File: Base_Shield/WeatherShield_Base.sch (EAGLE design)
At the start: 71 parts, among them Q1 BSS138, Q2 BSS138, U1 DS3231SN, U2 LT3652

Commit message: WeatherShield_v1
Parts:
- removed U$5: MCP3221A5T-E/OT, FSEWeatherShield:MCP3221A5T-E/OT
- added C5: 0.1uF, rcl:C-EUC0603
- added JP1, JP2, JP4: (no value), pinhead:PINHD-1X2
- added JP5: (no value), pinhead:PINHD-1X3
- added JP6, JP7, JP8: (no value), pinhead:PINHD-1X1
- added U3: TMP100MDBVREP, FSEWeatherShield:TMP100MDBVREP
- added U4: ADS1015IDGST, FSEWeatherShield:ADS1015IDGST
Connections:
- new net N$14: JP6.1, U4.AIN1
- new net N$18: JP4.1, PCB1.TXD0/GPIO14
- new net N$19: JP4.2, PCB1.RXD0/GPIO15
- new net N$20: JP5.3, PCB1.GPIO10/MOSI
- new net N$21: JP5.2, PCB1.GPIO09/MISO
- new net N$25: JP5.1, PCB1.GPIO11/SCLK
- new net N$8: JP7.1, U4.AIN2
- new net N$9: JP8.1, U4.AIN3
- net 3.3V: now also C5.1, JP2.1, U3.V+
- net 5V: now also JP1.1, U4.VDD; no longer C20.1, C21.1, U$5.VDD
- net GND: now also C5.2, JP1.2, JP2.2, U3.AD0, U3.AD1, U3.GND, U4.ADDR, U4.GND; no longer C20.2, C21.2, U$5.VSS
- net HV_SCL: now also U4.SCL; no longer PCB1.GPIO03/SCL1
- net HV_SDA: now also U4.SDA; no longer PCB1.GPIO02/SDA1
- net RAIN: now also PCB1.GPIO18
- net SCL: now also PCB1.GPIO03/SCL1, U3.SCL; no longer U$5.SCL
- net SDA: now also PCB1.GPIO02/SDA1, U3.SDA; no longer U$5.SDA
- net STAT3: now also PCB1.GPIO21
- net WDIR: now also U4.AIN0; no longer U$5.AIN
- net WSPEED: now also PCB1.GPIO17/GEN0
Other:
- note added: "7-Bit I2C Address is 0x48"
- note added: "7-Bit I2C Address is 0x68"
- note added: "Add. SPI"
- note added: "Add. UART"
- note added: "Air Board Interface"
- note added: "Level shifter"
- note added: "Solar cell"
- note added: "Temperatur sensor"
- moved on the sheet: C1, C10, C11, C12, C13, C14, C15, C16, C17, C18, C19, C2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

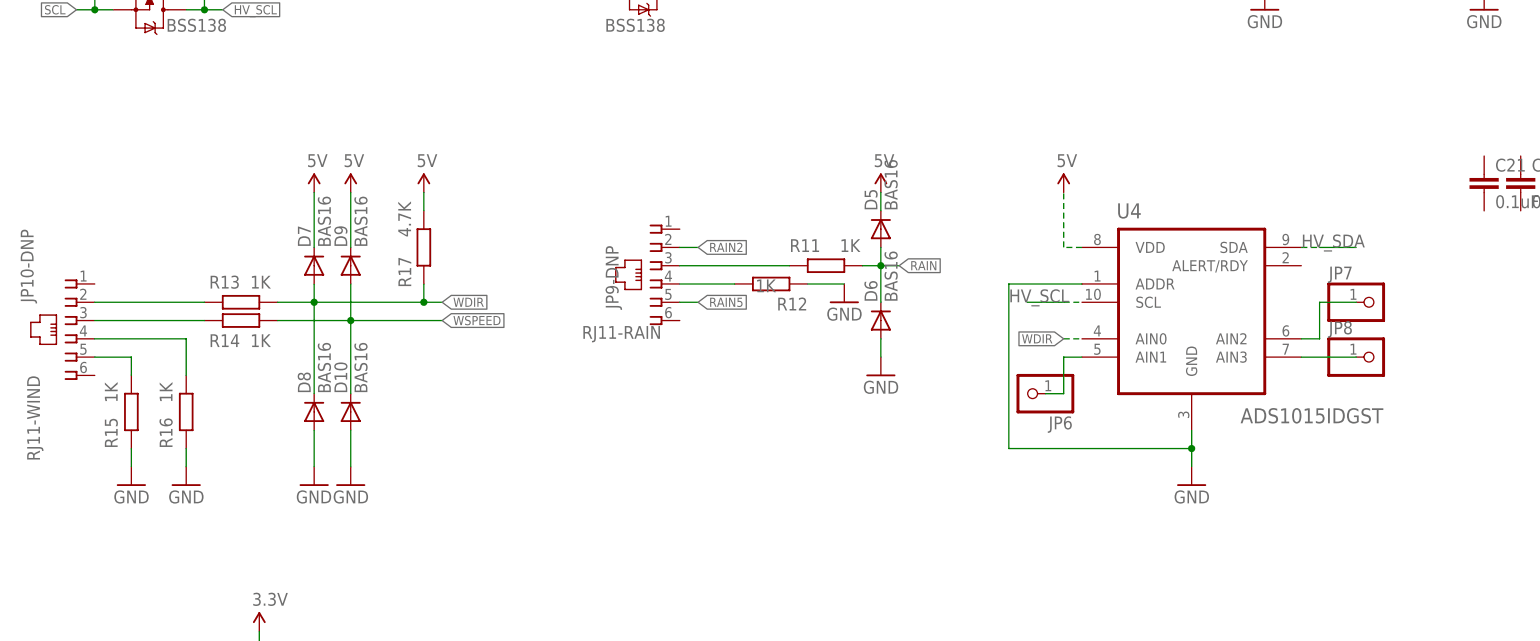
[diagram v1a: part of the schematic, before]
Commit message: WeatherShield_v1
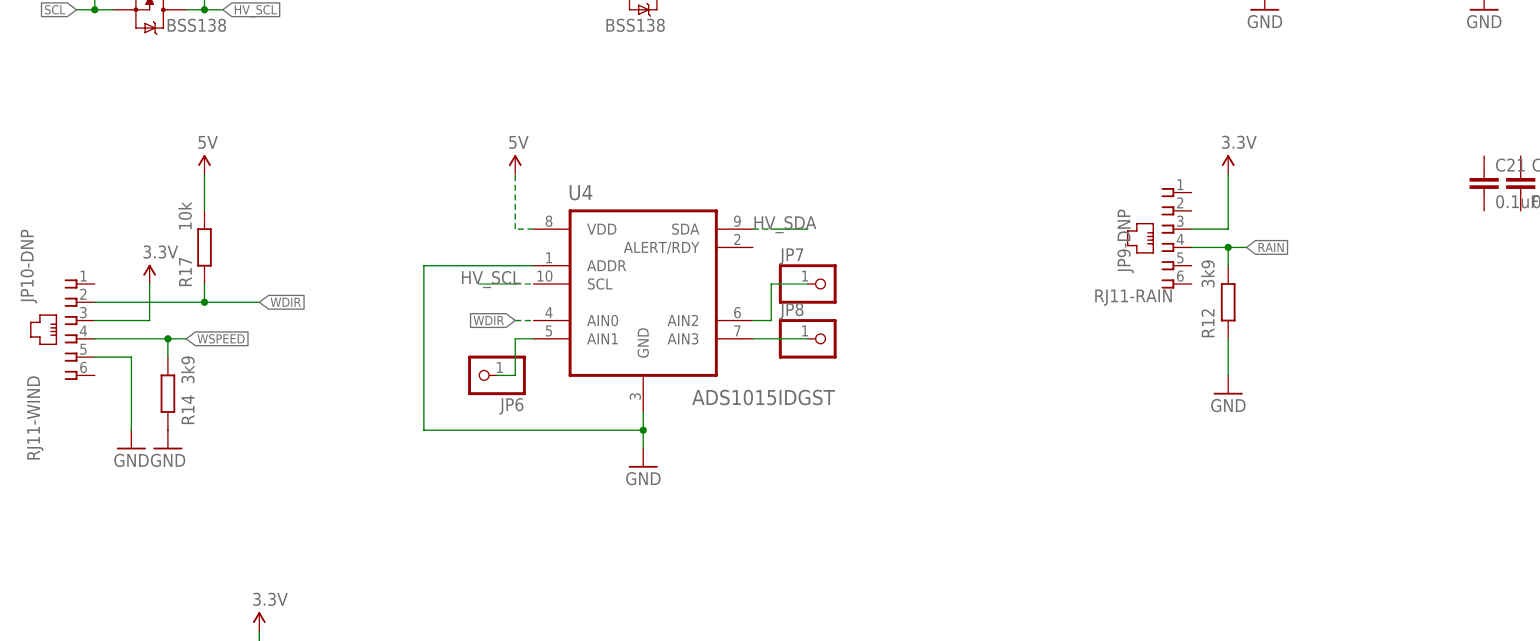
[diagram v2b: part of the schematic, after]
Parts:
- removed D10, D5, D6, D7, D8, D9: BAS16, SparkFun:DIODESOD
- removed R11, R13, R15, R16: 1K, rcl:R-EU_R0603
- R12, R14: value 1K -> 3k9
- R17: value 4.7K -> 10k
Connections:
- removed net N$1: JP10-DNP.3, R14.2
- removed net N$11: JP9-DNP.4, R12.1
- removed net N$12: JP10-DNP.5, R15.1
- removed net N$13: JP10-DNP.4, R16.1
- removed net N$2: JP10-DNP.2, R13.2
- removed net N$4: JP9-DNP.3, R11.2
- removed net RAIN2: JP9-DNP.2
- removed net RAIN5: JP9-DNP.5
- net 3.3V: now also JP10-DNP.3, JP9-DNP.3
- net 5V: no longer D5.C, D7.C, D9.C
- net GND: now also JP10-DNP.5, R14.2; no longer D10.A, D6.A, D8.A, R15.2, R16.2
- net RAIN: now also JP9-DNP.4, R12.1; no longer D5.A, D6.C, R11.1
- net WDIR: now also JP10-DNP.2; no longer D7.A, D8.C, R13.1
- net WSPEED: now also JP10-DNP.4; no longer D10.C, D9.A
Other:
- note added: "ADC 2 I2C"
- moved on the sheet: JP6, JP7, JP8, JP9-DNP, R12, R14, R17, U4
